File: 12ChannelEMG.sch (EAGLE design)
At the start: 47 parts

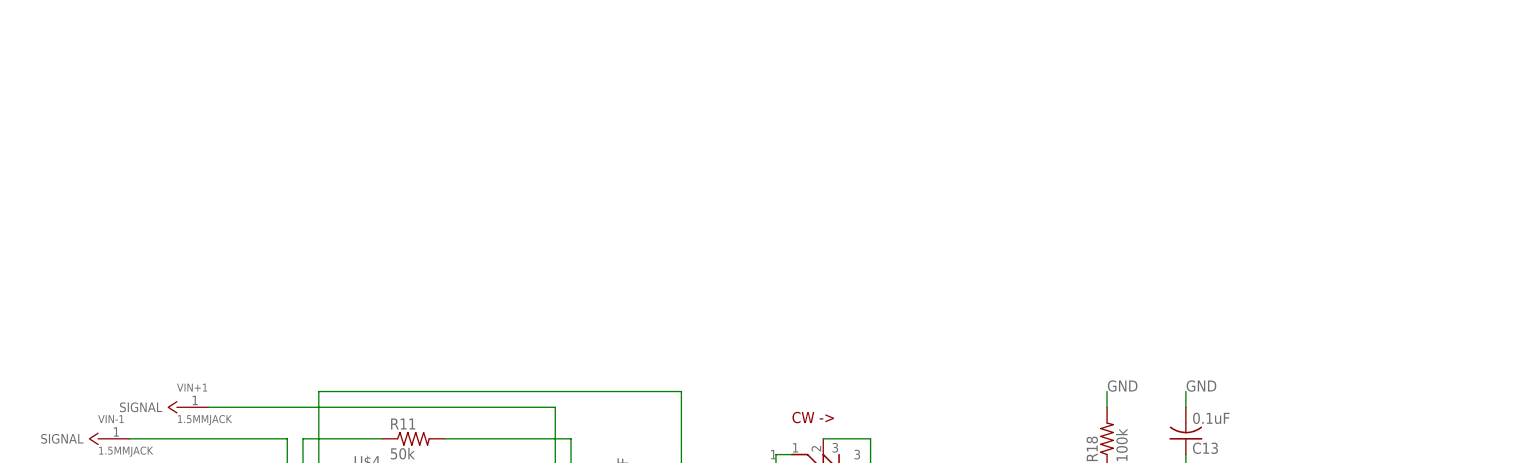
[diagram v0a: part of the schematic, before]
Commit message: Three Channels
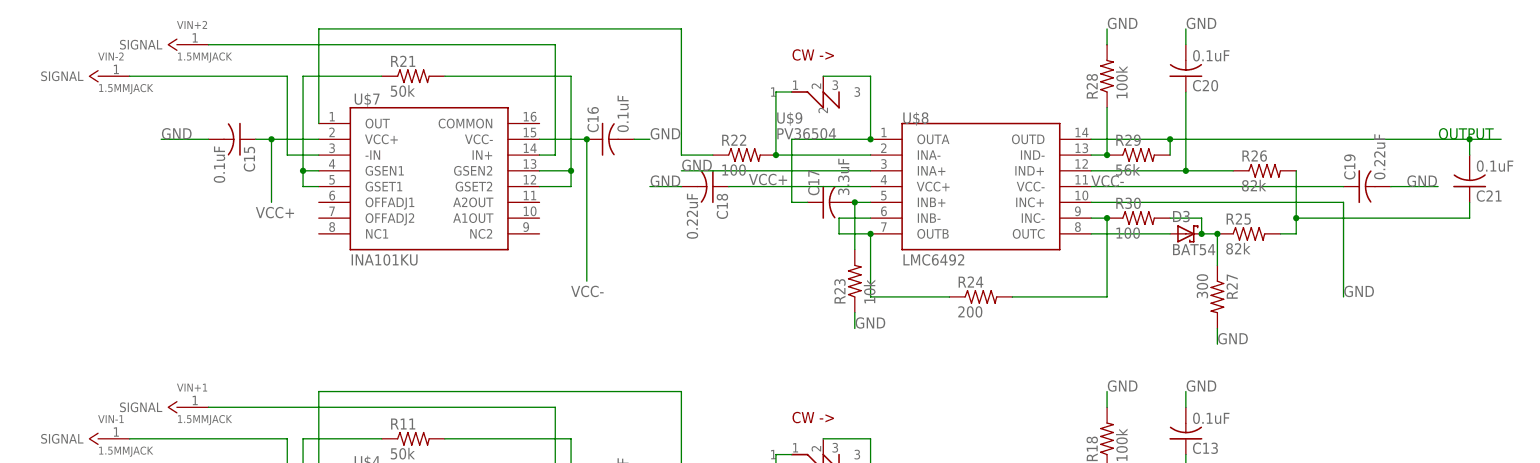
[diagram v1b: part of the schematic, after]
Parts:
- added C15, C16, C20, C21: 0.1uF, resistor:C-USC1206K
- added C17: 3.3uF, resistor:C-USC1206K
- added C18, C19: 0.22uF, rcl:C-USC0603K
- added D3: BAT54, diode:BAT54
- added R21: 50k, rcl:R-US_R0805
- added R22, R30: 100, resistor:R-US_R0603
- added R23: 10k, rcl:R-US_R0603
- added R24: 200, rcl:R-US_R0603
- added R25, R26: 82k, resistor:R-US_R0603
- added R27: 300, resistor:R-US_R0603
- added R28: 100k, resistor:R-US_R0603
- added R29: 56k, resistor:R-US_R0603
- added U$7: INA101KU, 12-ChannelEMG:INA101KUINA101KU
- added U$8: LMC6492, 12-ChannelEMG:LMC6492
- added U$9: PV36504, 12-ChannelEMG:PV36
- added VIN+2, VIN-2: 1.5MMJACK, 12-ChannelEMG:1.5MMJACK
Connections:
- new net N$35: R21.2, U$7.GSEN2, U$7.GSET2
- new net N$36: U$7.-IN, VIN-2.SIGNAL
- new net N$37: R22.2, U$8.INA-, U$9.1
- new net N$38: R22.1, U$7.OUT
- new net N$39: C17.1, U$8.OUTA, U$9.2
- new net N$40: C17.2, R23.2, U$8.INB+
- new net N$41: R24.1, U$8.INB-, U$8.OUTB
- new net N$42: R24.2, R30.1, U$8.INC-
- new net N$43: D3.A, U$8.OUTC
- new net N$44: C20.1, R26.1, U$8.IND+
- new net N$45: D3.C, R25.1, R27.1, R30.2
- new net N$46: C21.2, R29.2, U$8.OUTD
- new net N$47: R28.1, R29.1, U$8.IND-
- new net N$48: C21.1, R25.2, R26.2
- new net N$49: R21.1, U$7.GSEN1, U$7.GSET1
- new net N$50: U$7.IN+, VIN+2.SIGNAL
- net GND: now also C15.2, C16.2, C18.2, C19.2, C20.2, R23.1, R27.2, R28.2, U$8.INA+, U$8.INC+
- net VCC+: now also C15.1, C18.1, U$7.VCC+, U$8.VCC+
- net VCC-: now also C16.1, C19.1, U$7.VCC-, U$8.VCC-
